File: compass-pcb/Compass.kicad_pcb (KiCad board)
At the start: 2 copper layers, 6 parts

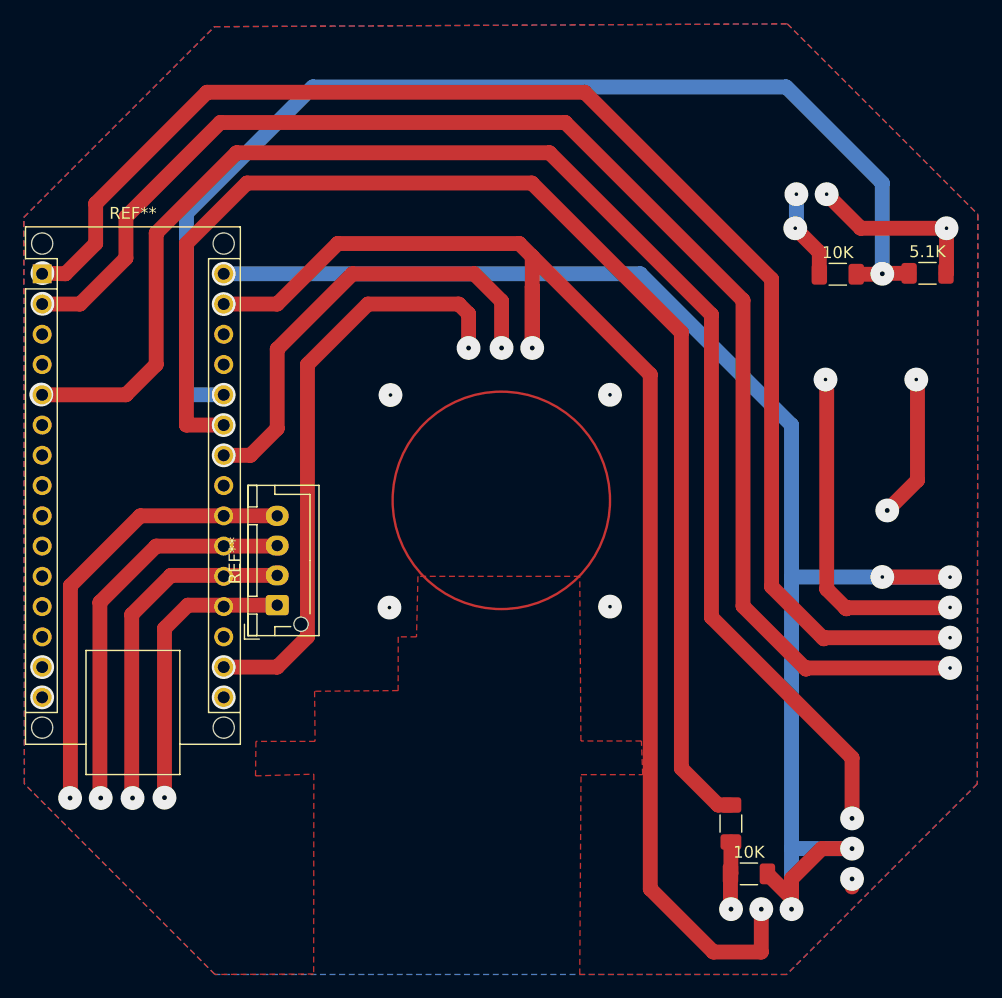
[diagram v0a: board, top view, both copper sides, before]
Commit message: adding comments to psb
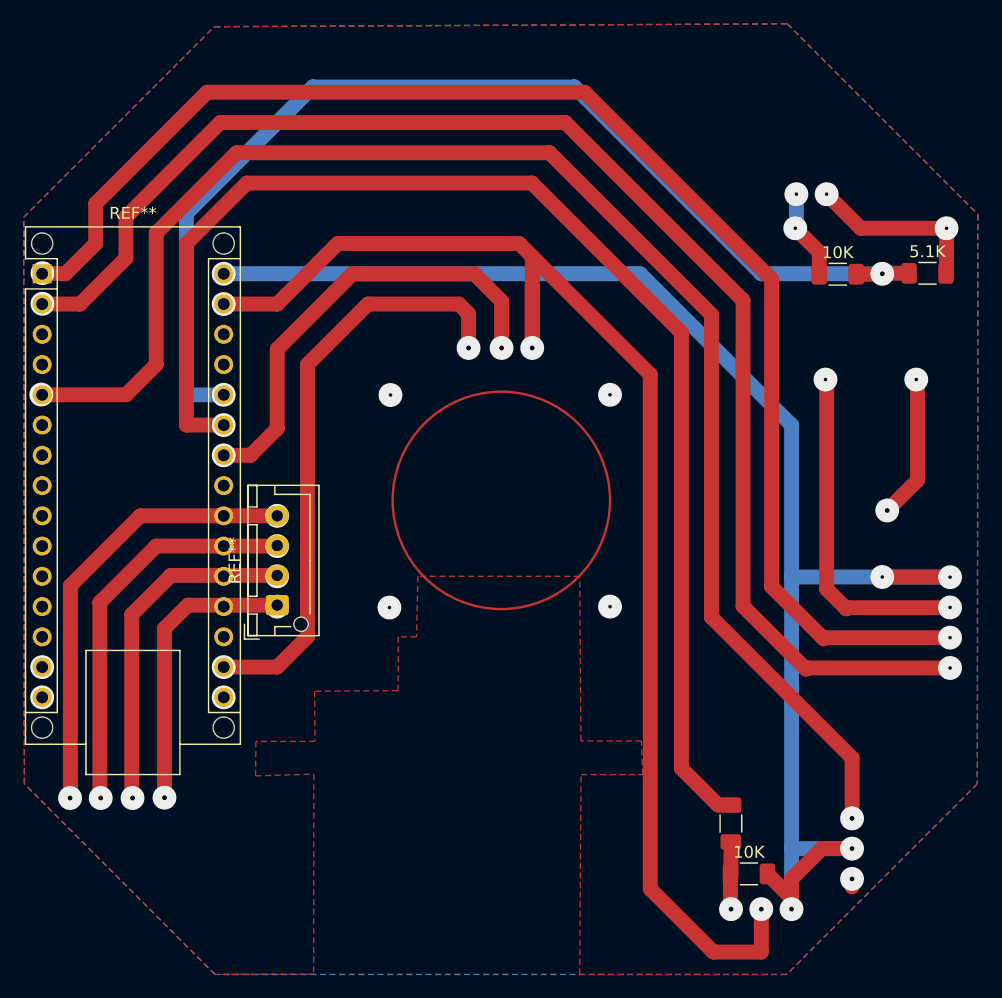
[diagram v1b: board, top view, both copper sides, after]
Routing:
- net (no net): track 950.9 -> 913.0 mm, vias 36 -> 38
- net GND: track 142.4 -> 175.8 mm, vias 6 -> 8
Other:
- board text added: "Battery"
- board text added: "Encoder"
- board text added: "GPS"
- board text added: "Hall Sensor (B)"
- board text added: "Power (charge/ discharge)"
- board text added: "Servo (A)"
